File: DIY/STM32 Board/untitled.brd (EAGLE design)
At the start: 100 x 80 mm, 13 parts, among them IC1 MCP1703DB, Q1 16 MHz, U1 STM32103RBT6

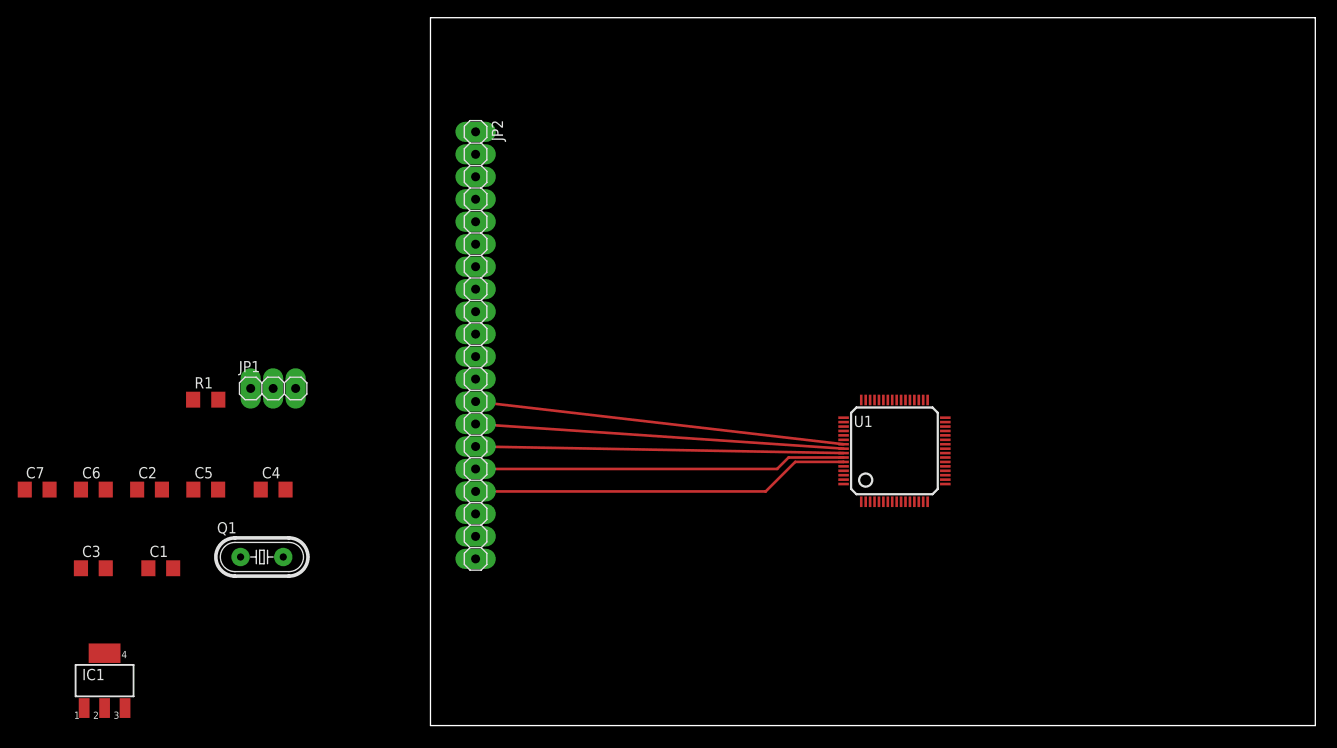
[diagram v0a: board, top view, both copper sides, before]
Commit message: DIY ++
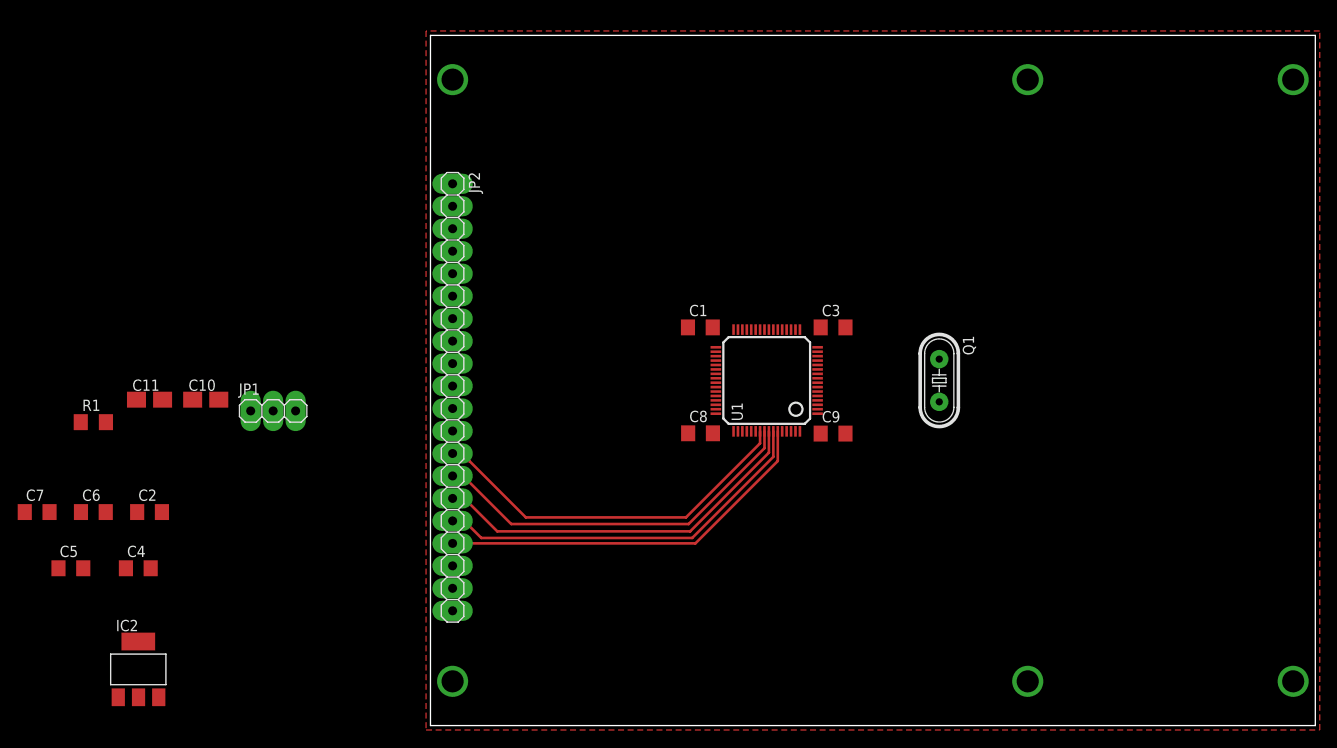
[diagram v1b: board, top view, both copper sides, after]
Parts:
- removed IC1: MCP1703DB, linear:SOT223
- added C10, C11: 10 uF, rcl:A/3216-18W
- added C8, C9: 100 nF, resistor:C1206
- added IC2: REG1117, burr-brown:SOT223
- moved C3 87.9 mm to (45.5, 45.0)
- moved Q1 79.1 mm to (57.5, 39.0), turned to 270 degrees
- moved C1 66.8 mm to (30.5, 45.0)
- moved C4 17.6 mm to (-33.0, 17.8)
- moved C5 17.6 mm to (-40.6, 17.8)
- moved U1 16.5 mm to (38.0, 39.0), turned to 90 degrees
- moved R1 13.0 mm to (-38.1, 34.3)
- moved JP2 6.42 mm to (2.50, 37.1)
- moved C2 2.54 mm to (-31.8, 24.1)
- moved C6 2.54 mm to (-38.1, 24.1)
- moved C7 2.54 mm to (-44.5, 24.1)
- moved JP1 2.54 mm to (-17.8, 35.6)
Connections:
- net +3V3: now also C1.2, C11.+, C9.1, IC2.2; no longer C1.1
- net +5V: now also C10.+, C8.2, IC2.3
- net GND: now also C1.1, C10.-, C11.-, C6.2, C7.2, C8.1, C9.2, IC2.1; no longer C1.2, C6.1, C7.1
- net N$1: now also C6.1; no longer C6.2
- net N$2: now also C7.1; no longer C7.2
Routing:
- net LCD_DB5: track 41.6 -> 43.4 mm
- net LCD_DB6: track 42.1 -> 43.7 mm
- net LCD_DB4: track 41.7 -> 43.0 mm
- net LCD_DB7: track 43.0 -> 44.0 mm
- net LCD_DB3: track 41.9 -> 42.6 mm
- added copper zone on layer 1, net GND
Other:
- board size 100 x 80 mm -> 100 x 78 mm
